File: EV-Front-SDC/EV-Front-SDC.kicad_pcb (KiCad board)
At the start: 2 copper layers, 78 x 58 mm, 28 parts, among them J1 JST-XA, J2 GPS, J2 JST-XA, J3 IMU, J3 JST-XA, J4 JST-XA, J5 JST-XA, J8 Conn_01x14, Q1 BSS205N, Q2 BSS205N, Q3 BSS205N, U2 MCP23S08-E_SS

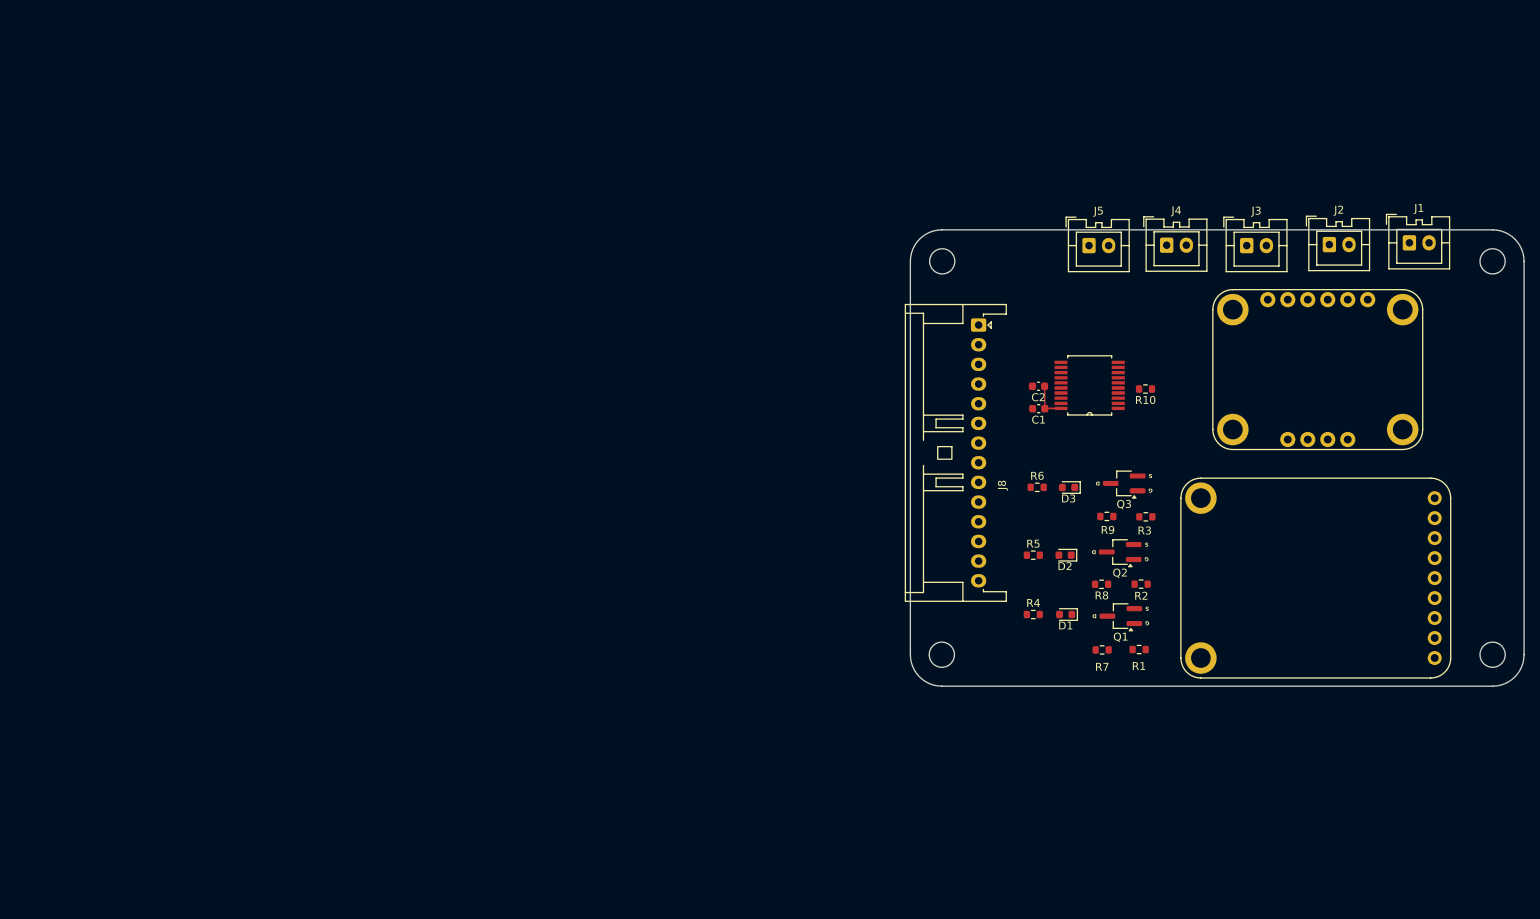
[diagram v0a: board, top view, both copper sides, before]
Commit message: Routed the PCB
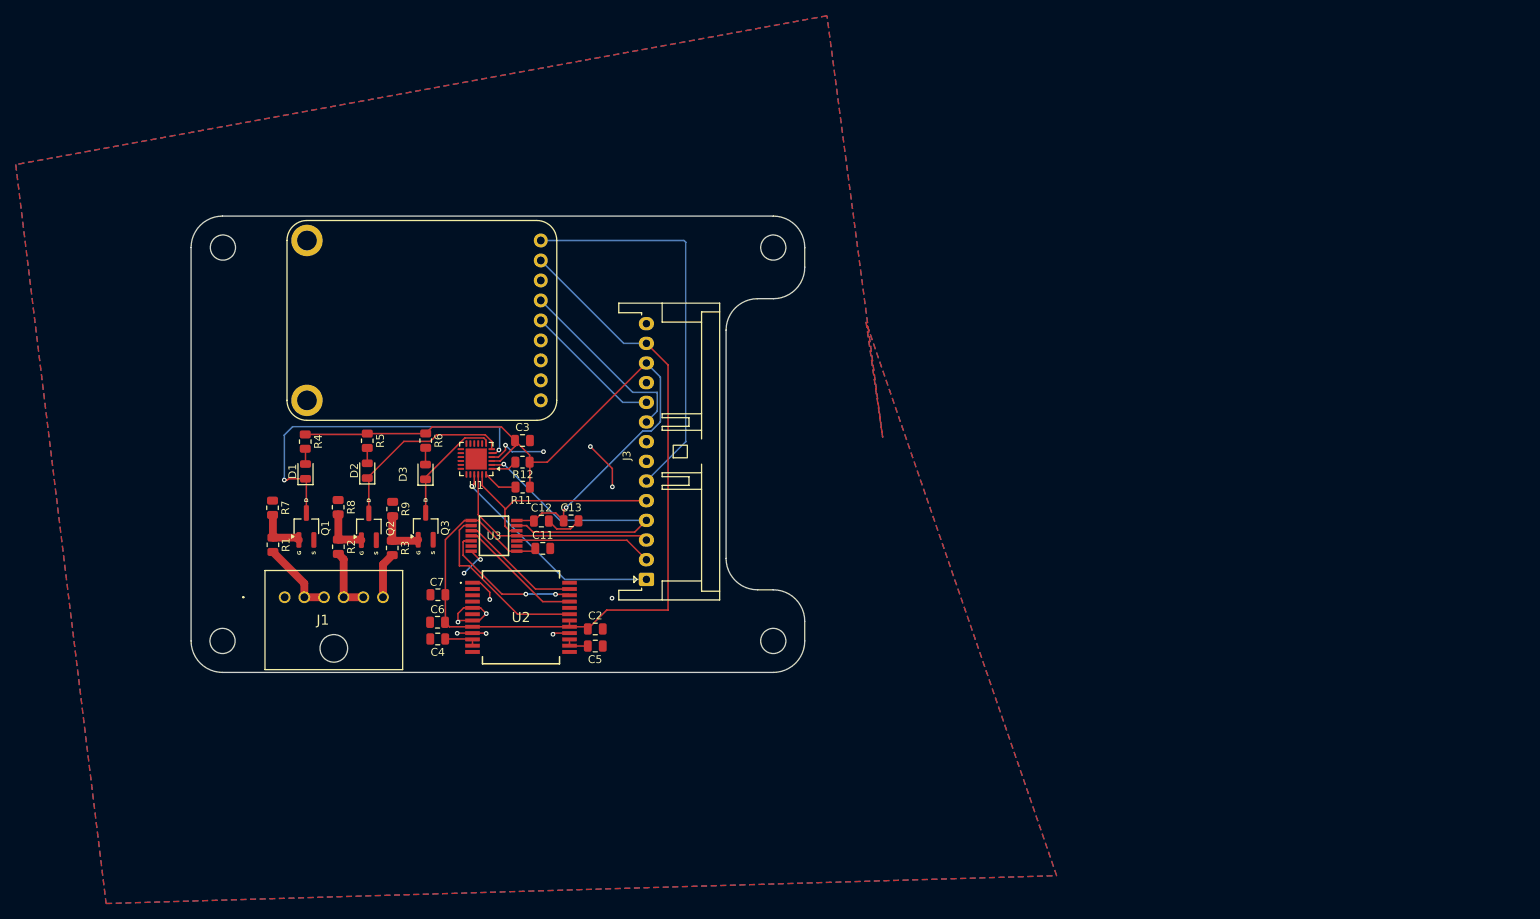
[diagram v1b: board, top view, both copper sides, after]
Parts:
- removed C1: 1u, Capacitor_SMD:C_0603_1608Metric
- removed the J2 at (186.8, 67.8)
- removed the J3 at (176.3, 67.9)
- removed J4, J5: JST-XA, Custom_MSM:Connector_JST-XA_2POS
- removed J8: Conn_01x14, Connector_JST:JST_XA_S14B-XASK-1_1x14_P2.50mm_Horizontal
- removed R10: 10k, Resistor_SMD:R_0603_1608Metric
- added C11: 0.1u, Capacitor_SMD:C_0805_2012Metric, F.Cu at (86.9, 106.4)
- added C12: 0.1u, Capacitor_SMD:C_0805_2012Metric, F.Cu at (86.7, 102.9)
- added C13: 1u, Capacitor_SMD:C_0805_2012Metric, F.Cu at (90.5, 102.9)
- added C3: 0.1u, Capacitor_SMD:C_0805_2012Metric, F.Cu at (84.3, 92.7)
- added C4: 10u, Capacitor_SMD:C_0805_2012Metric, F.Cu at (73.5, 117.9)
- added C5: 1u, Capacitor_SMD:C_0805_2012Metric, F.Cu at (93.5, 118.8)
- added C6: 1u, Capacitor_SMD:C_0805_2012Metric, F.Cu at (73.5, 115.8)
- added C7: 0.1u, Capacitor_SMD:C_0805_2012Metric, F.Cu at (73.5, 112.3)
- added R11: 10k, Resistor_SMD:R_0805_2012Metric, F.Cu at (84.3, 98.6)
- added R12: 10k, Resistor_SMD:R_0805_2012Metric, F.Cu at (84.3, 95.5)
- added U1: TXE8116DGSR, Package_DFN_QFN:QFN-24-1EP_4x4mm_P0.5mm_EP2.7x2.7mm, F.Cu at (78.4, 95.0)
- added U3: MAX3390EEUD_T, Custom_MSM:SOP65P640X110-14N, F.Cu at (80.7, 104.8)
- C2: footprint Capacitor_SMD:C_0603_1608Metric -> Capacitor_SMD:C_0805_2012Metric
- D1, D2, D3: footprint LED_SMD:LED_0603_1608Metric -> LED_SMD:LED_0805_2012Metric
- J1: value JST-XA -> B06B-PASK_LF__SN_; footprint Custom_MSM:Connector_JST-XA_2POS -> Custom_MSM:S06BXASK1LFSN
- J3: value IMU -> Conn_01x14; footprint CustomFootprints10:IMU -> Connector_JST:JST_XA_S14B-XASK-1_1x14_P2.50mm_Horizontal
- R1, R2, R3: value 40k -> 75K; footprint Resistor_SMD:R_0603_1608Metric -> Resistor_SMD:R_0805_2012Metric
- R4, R5, R6: footprint Resistor_SMD:R_0603_1608Metric -> Resistor_SMD:R_0805_2012Metric
- R7, R8, R9: value 10k -> 25k; footprint Resistor_SMD:R_0603_1608Metric -> Resistor_SMD:R_0805_2012Metric
- U2: value MCP23S08-E_SS -> SCH16T-K01-10; footprint Custom_MSM:SOP65P780X200-20N -> Custom_MSM:SCH16TK0110
- moved J1 149.9 mm to (54.1, 112.6)
- moved J2 118.2 mm to (75.3, 80.5)
- moved R1 110.9 mm to (52.6, 106.0), turned to -90 degrees
- moved R7 107.0 mm to (52.5, 101.3), turned to -90 degrees
- moved Q1 104.1 mm to (56.8, 103.6), turned to 90 degrees
- moved R2 102.1 mm to (60.9, 106.2), turned to -90 degrees
- moved D1 98.3 mm to (56.7, 96.6), turned to 90 degrees
- moved R8 97.5 mm to (60.9, 101.2), turned to -90 degrees
- moved R3 95.9 mm to (67.7, 106.4), turned to -90 degrees
- moved Q2 95.6 mm to (64.8, 103.7), turned to 90 degrees
- moved R4 95.1 mm to (56.7, 92.8), turned to -90 degrees
- moved REF** 91.4 mm to (81.2, 93.2)
- moved R9 90.8 mm to (67.8, 101.4), turned to -90 degrees
- moved D2 89.3 mm to (64.6, 96.5), turned to 90 degrees
- moved J3 89.2 mm to (100.0, 110.3), turned to 90 degrees
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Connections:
- C2 pad 1: +5V -> +3V3
- J1 pad 1: Net-(J1-Pin_1) -> Rear_SDC_In(Right)
- J3 pad 1: +3V3 -> 5V_CS_C
- J3 pad 10: unconnected-(J3-Pin_10-Pad10) -> TX
- J3 pad 2: unconnected-(J3-Pin_2-Pad2) -> 5V_CS_D
- J3 pad 3: GND -> 5V_SCLK
- J3 pad 4: SCL -> 5V_MISO
- J3 pad 5: SDA -> 5V_MOSI
- J3 pad 6: unconnected-(J3-Pin_6-Pad6) -> PPS
- J3 pad 9: unconnected-(J3-Pin_9-Pad9) -> RX
- U2 pad 1: 5V_SCLK -> GND
- U2 pad 10: unconnected-(U2-NC-Pad10) -> Net-(U2-VREGA)
- U2 pad 11: unconnected-(U2-NC-Pad10)_1 -> Net-(U2-VREGA)
- U2 pad 12: BOTS_S -> GND
- U2 pad 13: CK_S -> GND
- U2 pad 14: IS_S -> Net-(U2-VREGD)
- U2 pad 15: unconnected-(U2-GP3-Pad15) -> Net-(U2-VREGD)
- U2 pad 16: unconnected-(U2-GP4-Pad16) -> GND
- U2 pad 17: unconnected-(U2-GP5-Pad17) -> +3V3
- U2 pad 18: unconnected-(U2-GP6-Pad18) -> +3V3
- U2 pad 19: unconnected-(U2-GP7-Pad19) -> MISO
- U2 pad 2: 5V_MOSI -> unconnected-(U2-N.C.-Pad2)
- U2 pad 20: +5V -> unconnected-(U2-DRY_SYNC-Pad20)
- U2 pad 3: 5V_MISO -> unconnected-(U2-TA9-Pad3)
- U2 pad 4: +5V -> unconnected-(U2-TA8-Pad4)
- U2 pad 6: Net-(U2-~{RESET}) -> unconnected-(U2-EXTRESN-Pad6)
- U2 pad 7: 5V_CS_C -> GND
- U2 pad 8: unconnected-(U2-INT-Pad8) -> +3V3
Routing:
- net +3V3: track 0.00 -> 108.0 mm
- net +5V: track 4.95 -> 92.3 mm, vias 0 -> 1
- net PPS: track 0.00 -> 50.9 mm
- net BOTS_S: track 0.00 -> 44.8 mm, vias 0 -> 2
- net 5V_MISO: track 0.00 -> 40.1 mm, vias 0 -> 1
- net GND: track 0.00 -> 37.5 mm, vias 0 -> 13
- net 5V_CS_C: track 0.00 -> 28.7 mm, vias 0 -> 1
- net 5V_MOSI: track 0.00 -> 28.0 mm
- net 5V_SCLK: track 0.00 -> 27.9 mm
- net CK_S: track 0.00 -> 24.0 mm
- net RX: track 0.00 -> 24.0 mm
- net MISO: track 0.00 -> 22.8 mm
- net CS_D: track 0.00 -> 18.4 mm, vias 0 -> 2
- net TX: track 0.00 -> 17.7 mm
- net 5V_CS_D: track 0.00 -> 17.5 mm
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- added copper zone on B.Cu, net GND
- added copper zone on F.Cu, net GND
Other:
- outline, holes or cut-outs redrawn
